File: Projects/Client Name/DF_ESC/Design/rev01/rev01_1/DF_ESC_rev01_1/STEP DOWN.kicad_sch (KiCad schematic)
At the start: 0 parts

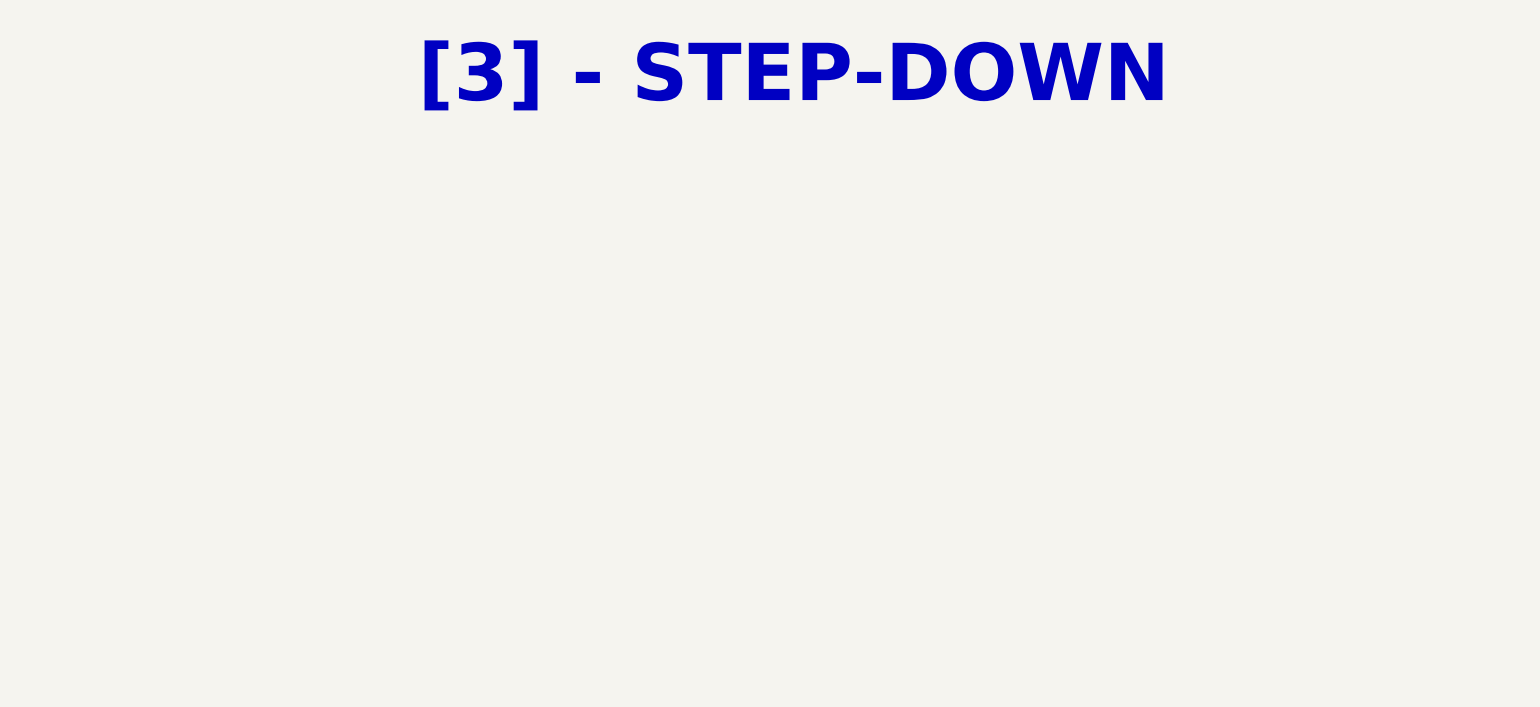
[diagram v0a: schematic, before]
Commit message: update 2024-02-29
CAN Page DONE
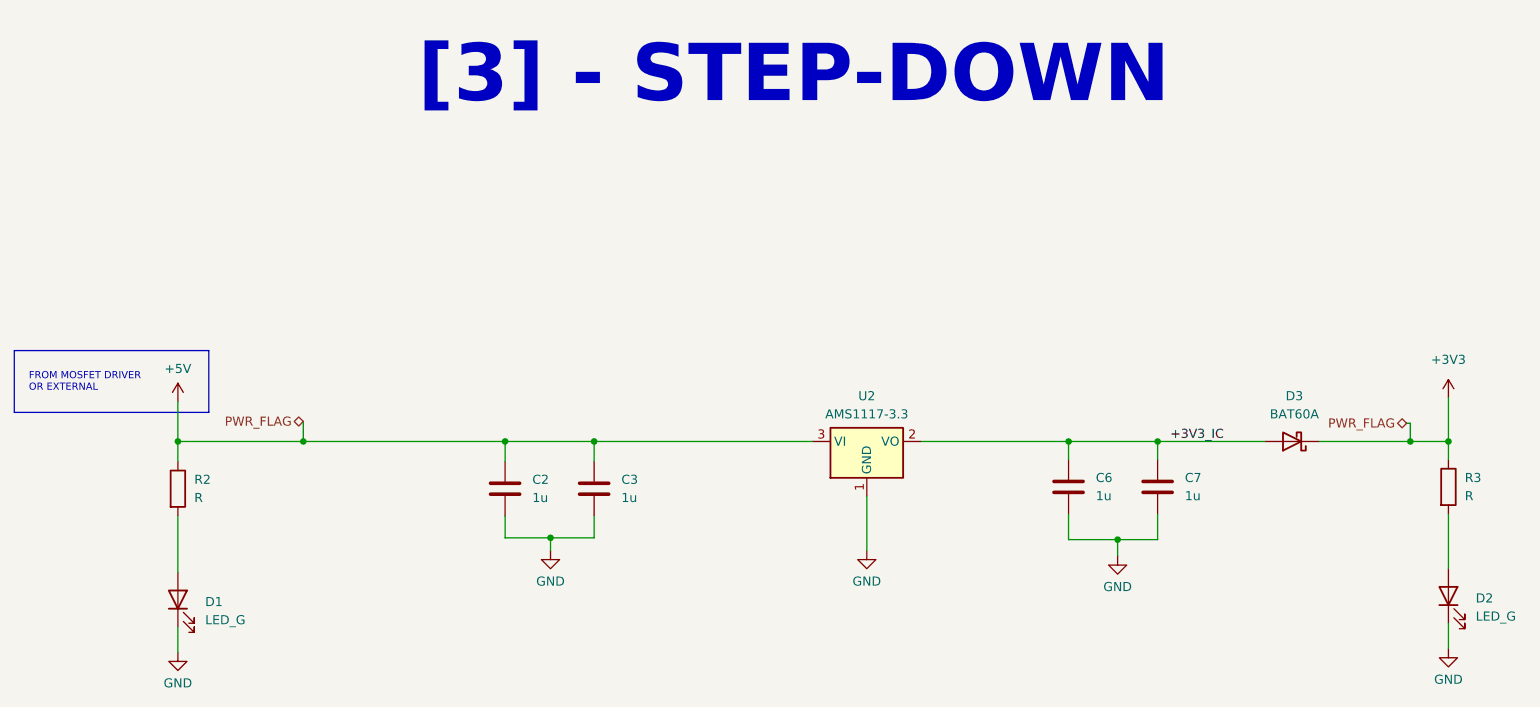
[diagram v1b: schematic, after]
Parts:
- added C2, C3, C6, C7: 1u, symbol Device:C
- added D1, D2: LED_G, symbol Device:LED
- added D3: BAT60A, Diode_SMD:D_SOD-323, symbol Diode:BAT60A
- added R2, R3: R, symbol Device:R
- added U2: AMS1117-3.3, Package_TO_SOT_SMD:SOT-223-3_TabPin2, symbol Regulator_Linear:AMS1117-3.3
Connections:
- new net: D1.2 (A), R2.2
- new net: D2.2 (A), R3.2
- new net +3V3: C2.1, C3.1, D3.1 (K), R2.1, R3.1, U2.3 (VI)
- new net +3V3_IC: C6.1, C7.1, D3.2 (A), U2.2 (VO)
- new net GND: C2.2, C3.2, C6.2, C7.2, D1.1 (K), D2.1 (K), U2.1 (GND)
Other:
- note added: "FROM MOSFET DRIVER OR EXTERNAL"
